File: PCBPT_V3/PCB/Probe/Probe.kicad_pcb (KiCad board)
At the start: 2 copper layers, 50 x 44 mm, 24 parts, among them IC1 VEML7700-TR, U1 SHT15, U2 MOUDLE-SEEEDUINO-XIAO

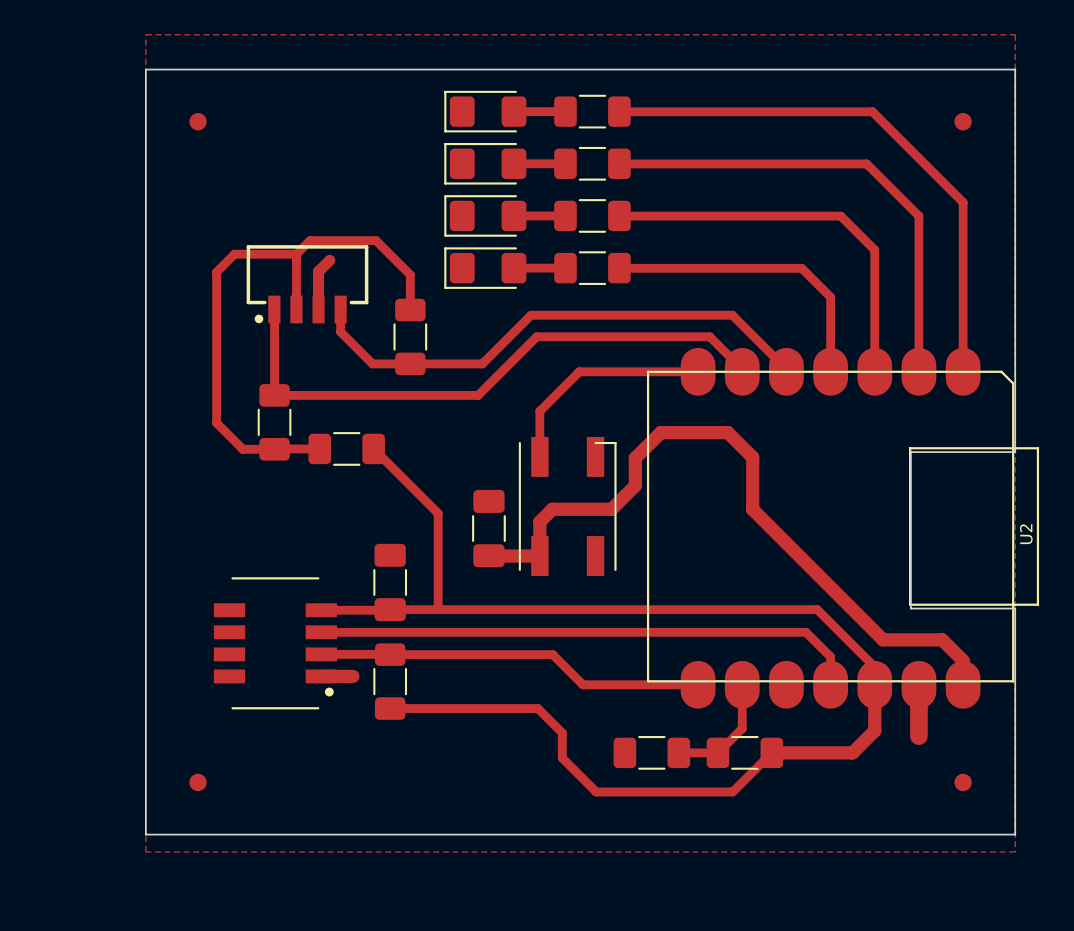
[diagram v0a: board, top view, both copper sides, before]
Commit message: udated by FZ
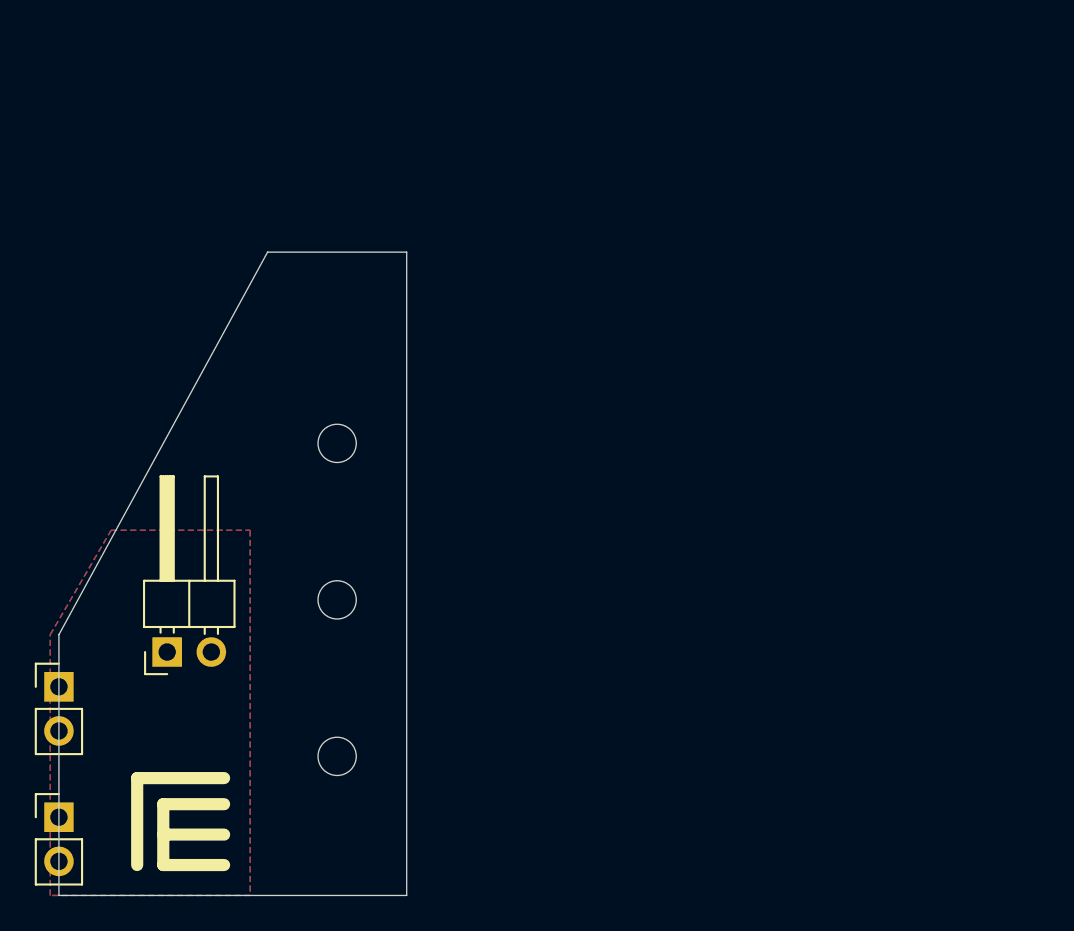
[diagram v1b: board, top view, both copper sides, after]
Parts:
- removed C1: 0.1uF, Capacitor_SMD:C_1206_3216Metric_Pad1.33x1.80mm_HandSolder
- removed C2: 10uF, Capacitor_SMD:C_1206_3216Metric_Pad1.33x1.80mm_HandSolder
- removed D1: SK6812, LED_SMD:LED_SK6812_PLCC4_5.0x5.0mm_P3.2mm
- removed D2, D3, D4, D5: R, LED_SMD:LED_1206_3216Metric_Pad1.42x1.75mm_HandSolder
- removed FID1, FID2, FID3, FID4: Fiducial, Fiducial:Fiducial_1mm_Mask2mm
- removed IC1: VEML7700-TR, SamacSys_Parts:VEML7700
- removed R1, R2, R3, R6: 200, Resistor_SMD:R_1206_3216Metric_Pad1.30x1.75mm_HandSolder
- removed R10: 0, Resistor_SMD:R_1206_3216Metric_Pad1.30x1.75mm_HandSolder
- removed R4, R5, R7, R8, R9: 10k, Resistor_SMD:R_1206_3216Metric_Pad1.30x1.75mm_HandSolder
- removed U1: SHT15, Mylib:DFN747X493X250-8N
- removed U2: MOUDLE-SEEEDUINO-XIAO, Mylib:MOUDLE14P-SMD-2.54-21X17.8MM
- added H1: MountingHole, MountingHole:MountingHole_2.2mm_M2, F.Cu at (136.0, 85.5)
- added H2: MountingHole, MountingHole:MountingHole_2.2mm_M2, F.Cu at (136.0, 94.5)
- added H3: MountingHole, MountingHole:MountingHole_2.2mm_M2, F.Cu at (136.0, 103.5)
- added J1: Conn_01x02_Pin, Connector_PinHeader_2.54mm:PinHeader_1x02_P2.54mm_Horizontal, F.Cu at (126.2, 97.5)
- added J2: Conn_01x02_Pin, Connector_PinHeader_2.54mm:PinHeader_1x02_P2.54mm_Vertical, F.Cu at (120.0, 107.0)
- added J3: Conn_01x02_Pin, Connector_PinHeader_2.54mm:PinHeader_1x02_P2.54mm_Vertical, F.Cu at (120.0, 99.5)
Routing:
- net +3V3: track 79.9 -> 0.00 mm
- net VBUS: track 40.9 -> 0.00 mm
- net /SCL: track 34.2 -> 0.00 mm
- net /PWR: track 33.1 -> 0.00 mm
- net /LED1: track 31.7 -> 0.00 mm
- net /SHT_CLK: track 31.5 -> 0.00 mm
- net /SDA: track 30.3 -> 0.00 mm
- net /LED2: track 27.4 -> 0.00 mm
- net /LED3: track 22.5 -> 0.00 mm
- net /SHT_DATA: track 22.4 -> 0.00 mm
- net /LED4: track 17.1 -> 0.00 mm
- net /DIN: track 12.7 -> 0.00 mm
- net GND: track 7.87 -> 0.00 mm
- net /A0: track 6.75 -> 0.00 mm
- net Net-(D5-A): track 2.96 -> 0.00 mm
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- added copper zone on B.Cu, net Net-(J1-Pin_1)
- added copper zone on F.Cu, net Net-(J1-Pin_1)
- removed copper zone on F.Cu, net GND
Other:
- board size 50 x 44 mm -> 20 x 37 mm
